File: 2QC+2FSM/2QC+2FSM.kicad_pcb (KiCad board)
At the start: 2 copper layers, 146.3 x 210.1 mm, 133 parts, among them J2 Screw_Terminal_01x04, U2 LM4040DBZ-2.0, U4 Teensy4.1, U7 LM4040DBZ-2.0, U8 LM4040DBZ-2.0, U9 LM4040DBZ-2.0, x1 TP_X1, x2 TP_X2, y1 TP_Y1, y2 TP_Y2

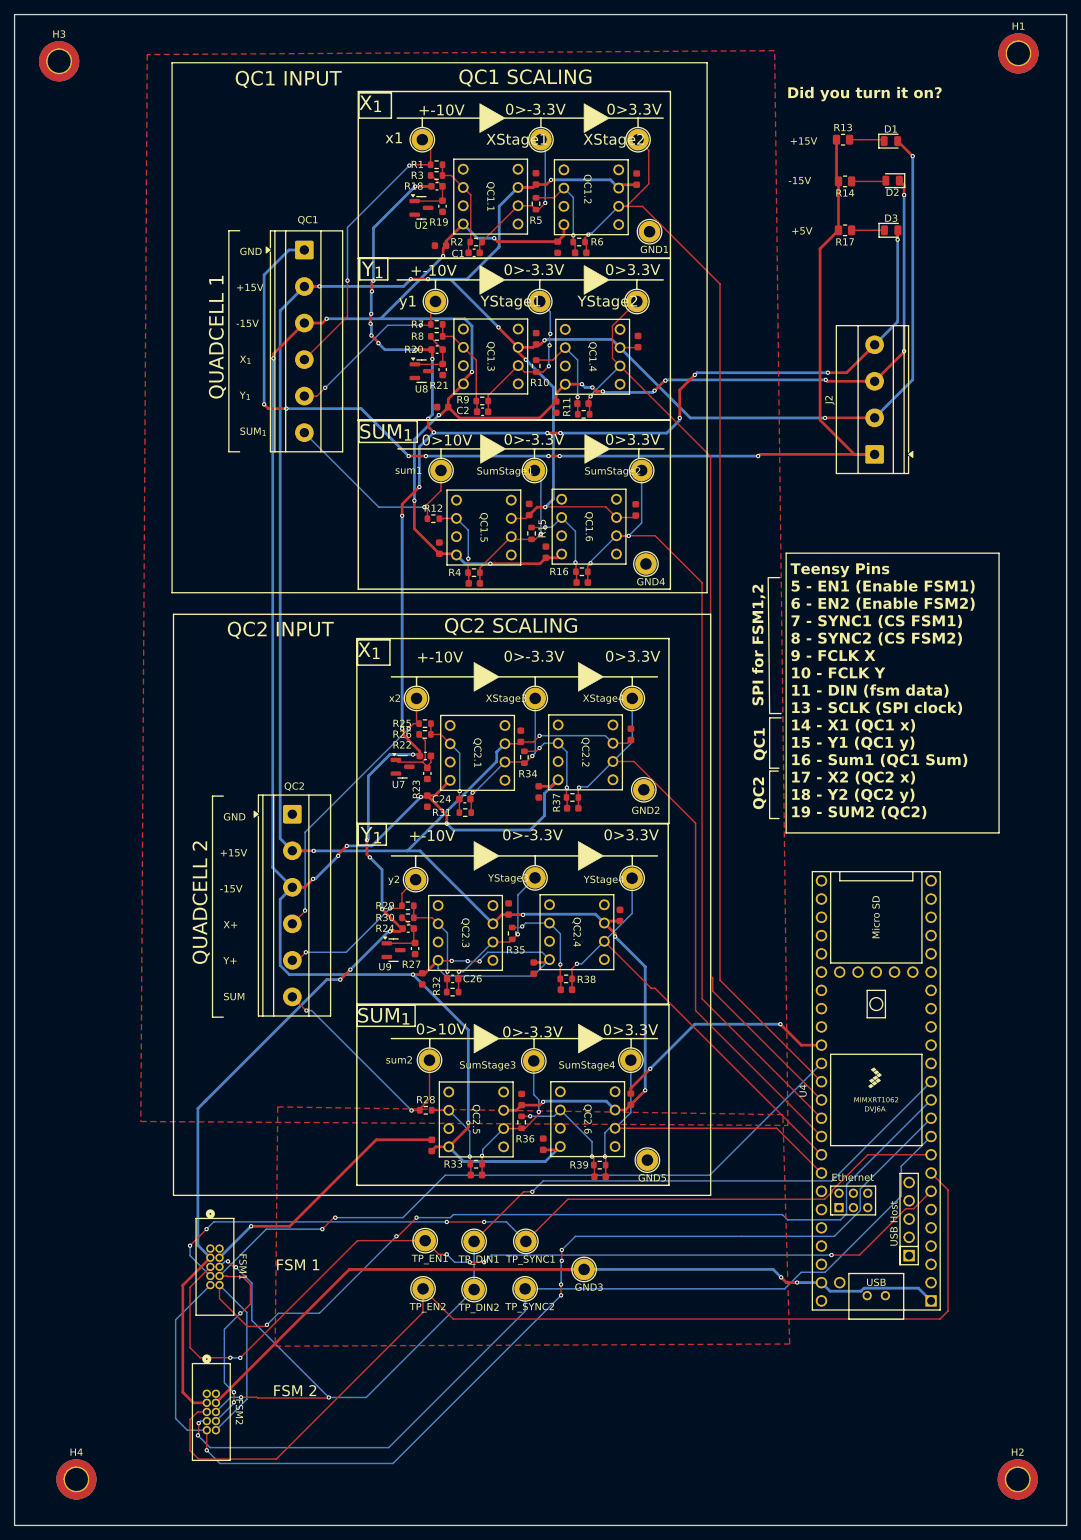
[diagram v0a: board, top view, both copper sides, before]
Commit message: added text and modified layout
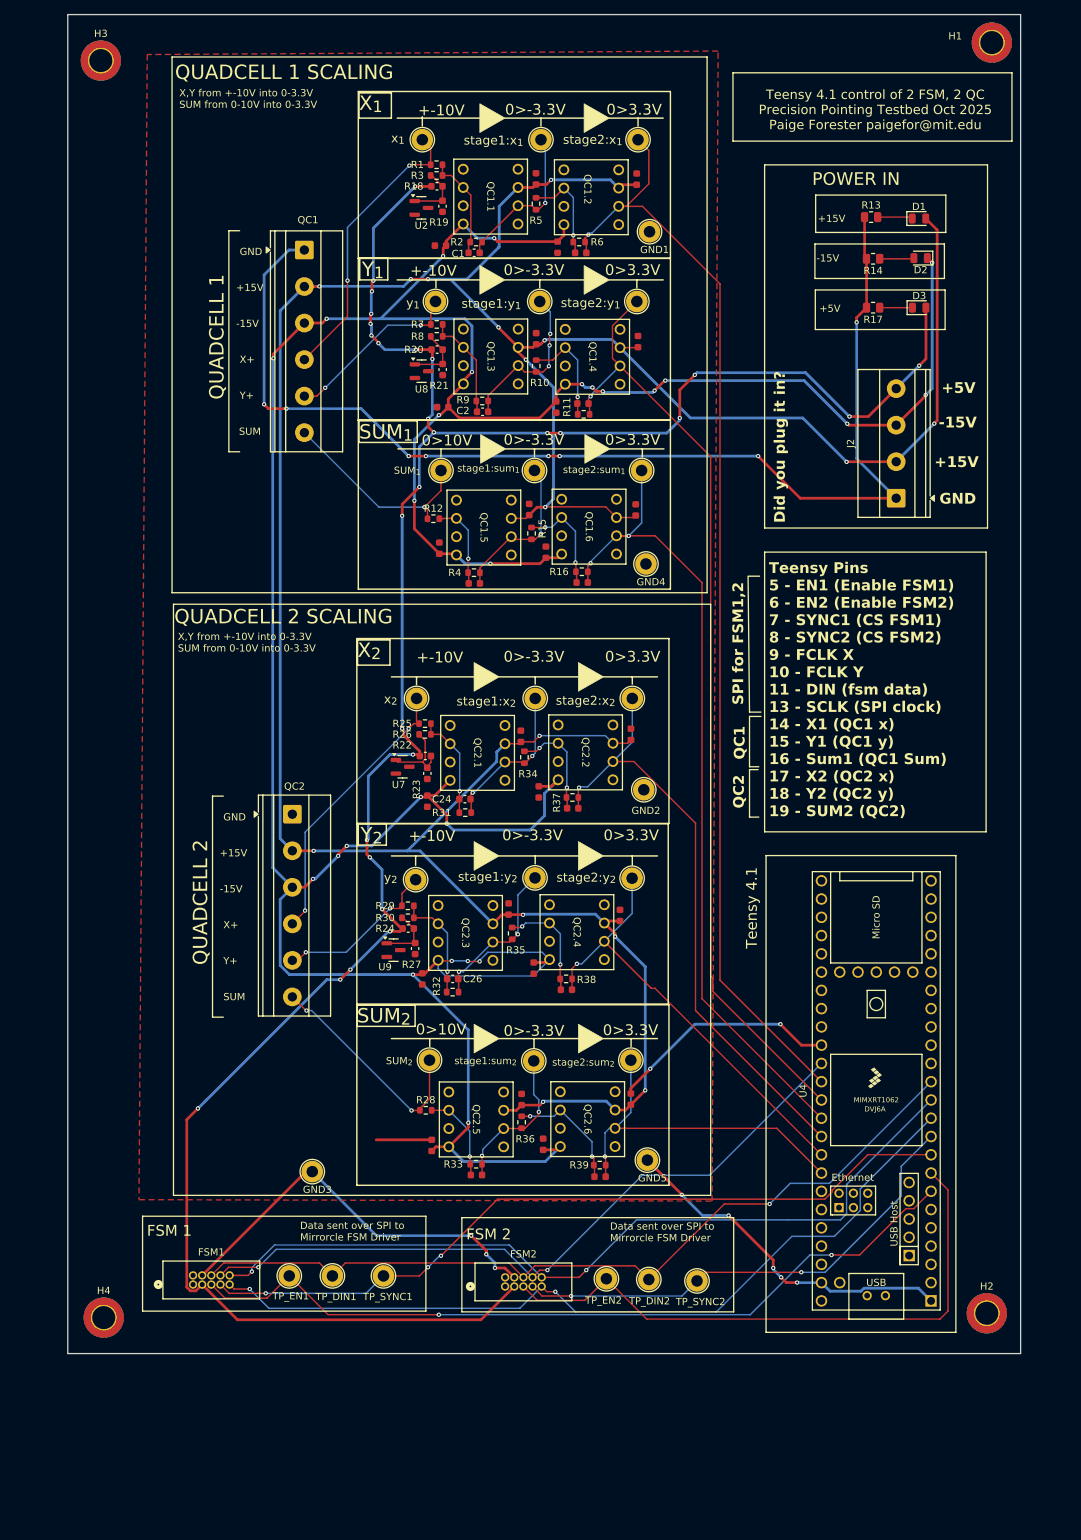
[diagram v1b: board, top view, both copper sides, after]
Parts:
- moved FSM2 44.1 mm to (116.0, 219.2), turned to 0 degrees
- moved GND3 40.2 mm to (89.2, 203.2)
- moved TP_EN2 25.5 mm to (130.1, 218.1)
- moved TP_DIN2 24.3 mm to (136.0, 218.2)
- moved TP_SYNC2 23.9 mm to (142.7, 218.4)
- moved H2 23.5 mm to (183.0, 222.9)
- moved H4 22.8 mm to (60.2, 223.5)
- moved TP_SYNC1 20.4 mm to (99.1, 217.7)
- moved TP_DIN1 20.3 mm to (92.0, 217.7)
- moved TP_EN1 19.5 mm to (86.0, 217.7)
- moved D3 11.4 mm to (173.6, 83.1)
- moved R13 11.4 mm to (166.9, 70.5)
- moved R14 11.4 mm to (167.2, 76.3)
- moved R17 11.4 mm to (167.2, 83.1)
- moved D1 11.4 mm to (173.6, 70.7)
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- renumbered x1 to x_{1}
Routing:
- net /EN2: track 147.1 -> 84.0 mm
- net /SYNC2: track 127.8 -> 67.6 mm
- net /FCLK_X: track 155.1 -> 114.5 mm, vias 5 -> 2
- net GND: track 340.5 -> 304.9 mm, vias 12 -> 18
- net /DIN: track 148.9 -> 116.0 mm, vias 5 -> 1
- net +5V: track 297.7 -> 328.6 mm, vias 27 -> 28
- net /FCLK_Y: track 142.0 -> 114.1 mm, vias 3 -> 2
- net /SCLK: track 122.9 -> 99.0 mm, vias 5 -> 2
- net /EN1: track 128.1 -> 111.5 mm, vias 6 -> 2
- net /SYNC1: track 116.0 -> 107.4 mm, vias 4 -> 3
- net -15V: track 468.9 -> 470.2 mm
- net +15V: track 429.9 -> 430.7 mm
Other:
- board size 146.3 x 210.1 mm -> 132.5 x 186.2 mm
- board text added: "Data sent over SPI to Mirrorcle FSM Driver"
- board text added: "Did you plug it in?"
- board text added: "POWER IN"
- board text added: "QUADCELL 1 SCALING"
- board text added: "QUADCELL 2 SCALING"
- board text added: "SUM_{2}"
- board text added: "Teensy 4.1"
- board text added: "Teensy 4.1 control of 2 FSM, 2 QC Precision Pointing Testbed Oct 2025 Paige Forester paigefor@mit.edu"
- board text added: "X,Y from +-10V into 0-3.3V SUM from 0-10V into 0-3.3V"
- board text added: "X_{2}"
- board text added: "Y_{2}"
- board text added: "stage1:sum_{1}"
- board text added: "stage1:sum_{2}"
- board text added: "stage1:x_{1}"
- board text added: "stage1:x_{2}"
- board text added: "stage1:y_{1}"
- board text added: "stage1:y_{2}"
- board text added: "stage2:sum_{1}"
- board text added: "stage2:sum_{2}"
- board text added: "stage2:x_{1}"
- board text added: "stage2:x_{2}"
- board text added: "stage2:y_{1}"
- board text added: "stage2:y_{2}"
- board text added: "x_{2}"
- board text added: "y_{1}"
- board text added: "y_{2}"
- board text removed: "Did you turn it on?"
- board text removed: "QC1 INPUT"
- board text removed: "QC1 SCALING"
- board text removed: "QC2 INPUT"
- board text removed: "QC2 SCALING"
